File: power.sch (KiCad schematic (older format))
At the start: 19 parts, among them P1 CONN_01X02, P2 CONN_01X02, P3 CONN_01X02, P4 CONN_01X02, U1 MC34063

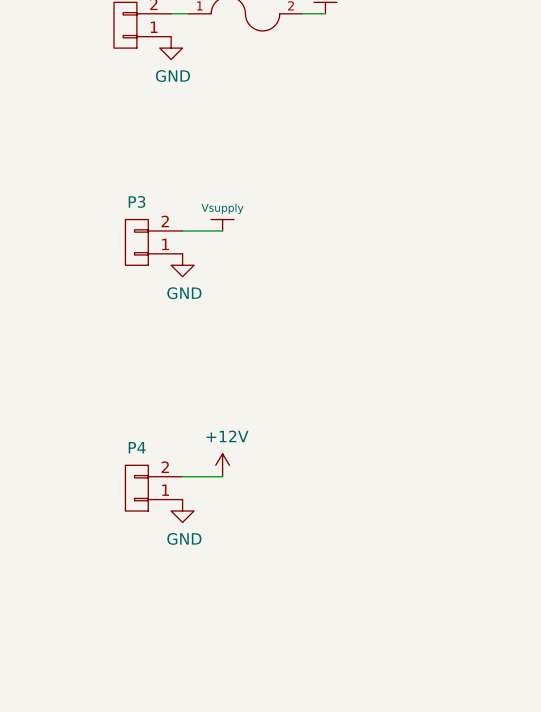
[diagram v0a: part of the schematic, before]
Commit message: Routing
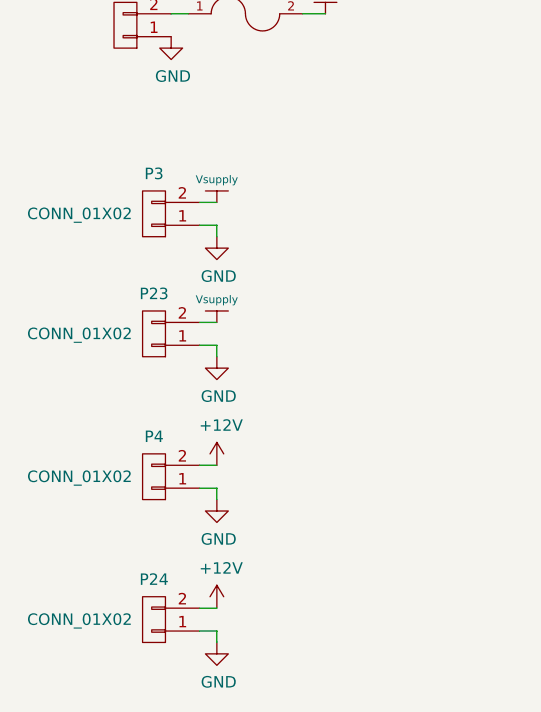
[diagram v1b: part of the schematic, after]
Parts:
- added P23, P24: CONN_01X02, headers:CON_HDR_1x2_2.54mm, symbol CONN_01X02
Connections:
- net +12V: now also P24.2 (P2)
- net GND: now also P23.1 (P1), P24.1 (P1)
- net Vsupply: now also P23.2 (P2)
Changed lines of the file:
@@
 $EndComp
 $Comp
-L +12V #PWR49
+L +12V #PWR15
 U 1 1 568AC408
 P 5150 1925
-F 0 "#PWR49" H 5150 1775 50  0001 C CNN
+F 0 "#PWR15" H 5150 1775 50  0001 C CNN
 F 1 "+12V" H 5168 2099 50  0000 C CNN
 F 2 "" H 5150 1925 50  0000 C CNN
@@
 $EndComp
 $Comp
-L GND #PWR4
+L GND #PWR6
 U 1 1 568AE875
 P 1425 4450
-F 0 "#PWR4" H 1425 4200 50  0001 C CNN
+F 0 "#PWR6" H 1425 4200 50  0001 C CNN
 F 1 "GND" H 1433 4276 50  0000 C CNN
 F 2 "" H 1425 4450 50  0000 C CNN
@@
 $EndComp
 $Comp
-L GND #PWR23
+L GND #PWR14
 U 1 1 568AE8A5
 P 2800 2325
-F 0 "#PWR23" H 2800 2075 50  0001 C CNN
+F 0 "#PWR14" H 2800 2075 50  0001 C CNN
 F 1 "GND" H 2808 2151 50  0000 C CNN
 F 2 "" H 2800 2325 50  0000 C CNN
@@
 	1500 4350 1425 4350
 $Comp
-L Vsupply #P11
+L Vsupply #P6
 U 1 1 568AD53F
 P 4750 1225
-F 0 "#P11" H 4750 1225 60  0001 C CNN
+F 0 "#P6" H 4750 1225 60  0001 C CNN
 F 1 "Vsupply" H 4750 1175 34  0000 C CNN
 F 2 "" H 4750 1225 60  0000 C CNN
@@
 $EndComp
 $Comp
-L GND #PWR6
+L GND #PWR7
 U 1 1 568ADBA9
 P 1450 3800
-F 0 "#PWR6" H 1450 3550 50  0001 C CNN
+F 0 "#PWR7" H 1450 3550 50  0001 C CNN
 F 1 "GND" H 1458 3626 50  0000 C CNN
 F 2 "" H 1450 3800 50  0000 C CNN
@@
 	1525 3700 1450 3700
 $Comp
-L Vsupply #P4
+L Vsupply #P5
 U 1 1 568ADC9C
 P 2125 3550
-F 0 "#P4" H 2125 3550 60  0001 C CNN
+F 0 "#P5" H 2125 3550 60  0001 C CNN
 F 1 "Vsupply" H 2125 3500 34  0000 C CNN
 F 2 "" H 2125 3550 60  0000 C CNN
@@
 $EndComp
 $Comp
-L Vheatbed #P3
+L Vheatbed #P4
 U 1 1 568AE31D
 P 2100 4200
-F 0 "#P3" H 2100 4200 60  0001 C CNN
+F 0 "#P4" H 2100 4200 60  0001 C CNN
 F 1 "Vheatbed" H 2100 4150 34  0000 C CNN
 F 2 "" H 2100 4200 60  0000 C CNN
@@
 	1    0    0    -1
 $EndComp
+Connection ~ 2025 1725
+$Comp
+L GND #PWR8
+U 1 1 56BC5BCA
+P 1625 5325
+F 0 "#PWR8" H 1625 5075 50  0001 C CNN
+F 1 "GND" H 1633 5151 50  0000 C CNN
+F 2 "" H 1625 5325 50  0000 C CNN
+F 3 "" H 1625 5325 50  0000 C CNN
+	1    1625 5325
+	1    0    0    -1
+$EndComp
+Wire Wire Line
+	1550 5175 1625 5175
+Wire Wire Line
+	1550 5275 1625 5275
+Wire Wire Line
+	1625 5275 1625 5325
+$Comp
+L Vsupply #P2
+U 1 1 56BC5C4C
+P 1625 5025
+F 0 "#P2" H 1625 5025 60  0001 C CNN
+F 1 "Vsupply" H 1625 4975 34  0000 C CNN
+F 2 "" H 1625 5025 60  0000 C CNN
+F 3 "" H 1625 5025 60  0000 C CNN
+	1    1625 5025
+	1    0    0    -1
+$EndComp
 $Comp
 L CONN_01X02 P3
-U 1 1 568AE687
-P 1275 5350
-F 0 "P3" H 1275 5175 50  0000 C CNN
-F 1 "CONN_01X02" H 1194 5160 50  0001 C CNN
-F 2 "headers:CON_HDR_1x2_2.54mm" H 1275 5350 50  0001 C CNN
-F 3 "" H 1275 5350 50  0000 C CNN
-	1    1275 5350
-	-1   0    0    1
+U 1 1 56BC61F9
+P 1350 5225
+F 0 "P3" H 1350 5050 50  0000 C CNN
+F 1 "CONN_01X02" H 1675 5225 50  0000 C CNN
+F 2 "headers:CON_HDR_1x2_2.54mm" H 1350 5225 50  0001 C CNN
+F 3 "" H 1350 5225 50  0000 C CNN
+	1    1350 5225
+	-1   0    0    1
+$EndComp
+$Comp
+L GND #PWR11
+U 1 1 56BC656B
+P 1625 6475
+F 0 "#PWR11" H 1625 6225 50  0001 C CNN
+F 1 "GND" H 1633 6301 50  0000 C CNN
+F 2 "" H 1625 6475 50  0000 C CNN
+F 3 "" H 1625 6475 50  0000 C CNN
+	1    1625 6475
+	1    0    0    -1
+$EndComp
+Wire Wire Line
+	1550 6325 1625 6325
+Wire Wire Line
+	1550 6425 1625 6425
+Wire Wire Line
+	1625 6425 1625 6475
+$Comp
+L CONN_01X02 P4
+U 1 1 56BC657A
+P 1350 6375
+F 0 "P4" H 1350 6200 50  0000 C CNN
+F 1 "CONN_01X02" H 1675 6375 50  0000 C CNN
+F 2 "headers:CON_HDR_1x2_2.54mm" H 1350 6375 50  0001 C CNN
+F 3 "" H 1350 6375 50  0000 C CNN
+	1    1350 6375
+	-1   0    0    1
+$EndComp
+$Comp
+L +12V #PWR10
+U 1 1 56BC66FC
+P 1625 6325
+F 0 "#PWR10" H 1625 6175 50  0001 C CNN
+F 1 "+12V" H 1643 6499 50  0000 C CNN
+F 2 "" H 1625 6325 50  0000 C CNN
+F 3 "" H 1625 6325 50  0000 C CNN
+	1    1625 6325
+	1    0    0    -1
 $EndComp
 $Comp
 L GND #PWR9
-U 1 1 568AE68D
-P 1475 5400
-F 0 "#PWR9" H 1475 5150 50  0001 C CNN
-F 1 "GND" H 1483 5226 50  0000 C CNN
-F 2 "" H 1475 5400 50  0000 C CNN
-F 3 "" H 1475 5400 50  0000 C CNN
-	1    1475 5400
-	1    0    0    -1
-$EndComp
-Wire Wire Line
-	1475 5300 1650 5300
-$Comp
-L Vsupply #P2
-U 1 1 568AE69B
-P 1650 5150
-F 0 "#P2" H 1650 5150 60  0001 C CNN
-F 1 "Vsupply" H 1650 5100 34  0000 C CNN
-F 2 "" H 1650 5150 60  0000 C CNN
-F 3 "" H 1650 5150 60  0000 C CNN
-	1    1650 5150
-	1    0    0    -1
-$EndComp
-$Comp
-L CONN_01X02 P4
-U 1 1 568AE85A
-P 1275 6425
-F 0 "P4" H 1275 6250 50  0000 C CNN
-F 1 "CONN_01X02" H 1194 6235 50  0001 C CNN
-F 2 "headers:CON_HDR_1x2_2.54mm" H 1275 6425 50  0001 C CNN
-F 3 "" H 1275 6425 50  0000 C CNN
-	1    1275 6425
-	-1   0    0    1
-$EndComp
-$Comp
-L GND #PWR10
-U 1 1 568AE860
-P 1475 6475
-F 0 "#PWR10" H 1475 6225 50  0001 C CNN
-F 1 "GND" H 1483 6301 50  0000 C CNN
-F 2 "" H 1475 6475 50  0000 C CNN
-F 3 "" H 1475 6475 50  0000 C CNN
-	1    1475 6475
-	1    0    0    -1
-$EndComp
-Wire Wire Line
-	1475 6375 1650 6375
-$Comp
-L +12V #PWR11
-U 1 1 568BD457
-P 1650 6375
-F 0 "#PWR11" H 1650 6225 50  0001 C CNN
-F 1 "+12V" H 1668 6549 50  0000 C CNN
-F 2 "" H 1650 6375 50  0000 C CNN
-F 3 "" H 1650 6375 50  0000 C CNN
-	1    1650 6375
-	1    0    0    -1
-$EndComp
-Connection ~ 2025 1725
+U 1 1 56BC6A92
+P 1625 5850
+F 0 "#PWR9" H 1625 5600 50  0001 C CNN
+F 1 "GND" H 1633 5676 50  0000 C CNN
+F 2 "" H 1625 5850 50  0000 C CNN
+F 3 "" H 1625 5850 50  0000 C CNN
+	1    1625 5850
+	1    0    0    -1
+$EndComp
+Wire Wire Line
+	1550 5700 1625 5700
+Wire Wire Line
+	1550 5800 1625 5800
+Wire Wire Line
+	1625 5800 1625 5850
+$Comp
+L Vsupply #P3
+U 1 1 56BC6A9B
+P 1625 5550
+F 0 "#P3" H 1625 5550 60  0001 C CNN
+F 1 "Vsupply" H 1625 5500 34  0000 C CNN
+F 2 "" H 1625 5550 60  0000 C CNN
+F 3 "" H 1625 5550 60  0000 C CNN
+	1    1625 5550
+	1    0    0    -1
+$EndComp
+$Comp
+L CONN_01X02 P23
+U 1 1 56BC6AA1
+P 1350 5750
+F 0 "P23" H 1350 5575 50  0000 C CNN
+F 1 "CONN_01X02" H 1675 5750 50  0000 C CNN
+F 2 "headers:CON_HDR_1x2_2.54mm" H 1350 5750 50  0001 C CNN
+F 3 "" H 1350 5750 50  0000 C CNN
+	1    1350 5750
+	-1   0    0    1
+$EndComp
+$Comp
+L GND #PWR13
+U 1 1 56BC6B73
+P 1625 7100
+F 0 "#PWR13" H 1625 6850 50  0001 C CNN
+F 1 "GND" H 1633 6926 50  0000 C CNN
+F 2 "" H 1625 7100 50  0000 C CNN
+F 3 "" H 1625 7100 50  0000 C CNN
+	1    1625 7100
+	1    0    0    -1
+$EndComp
+Wire Wire Line
+	1550 6950 1625 6950
+Wire Wire Line
+	1550 7050 1625 7050
+Wire Wire Line
+	1625 7050 1625 7100
+$Comp
+L CONN_01X02 P24
+U 1 1 56BC6B7C
+P 1350 7000
+F 0 "P24" H 1350 6825 50  0000 C CNN
+F 1 "CONN_01X02" H 1675 7000 50  0000 C CNN
+F 2 "headers:CON_HDR_1x2_2.54mm" H 1350 7000 50  0001 C CNN
+F 3 "" H 1350 7000 50  0000 C CNN
+	1    1350 7000
+	-1   0    0    1
+$EndComp
+$Comp
+L +12V #PWR12
+U 1 1 56BC6B82
+P 1625 6950
+F 0 "#PWR12" H 1625 6800 50  0001 C CNN
+F 1 "+12V" H 1643 7124 50  0000 C CNN
+F 2 "" H 1625 6950 50  0000 C CNN
+F 3 "" H 1625 6950 50  0000 C CNN
+	1    1625 6950
+	1    0    0    -1
+$EndComp
 $EndSCHEMATC
